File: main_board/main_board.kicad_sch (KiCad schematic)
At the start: 77 parts, among them J1 3.5mm Jack, J18 Conn_01x15_Female, J19 Conn_01x15_Female, J2 3.5mm Jack, J20 Conn_01x02_Male, J3 3.5mm Jack, J4 3.5mm Jack, J5 Display Header, J6 EU Power, J7 Expansion Header, SW1 Push Button, SW10 Push Button, SW11 Push Button, SW12 Push Button, SW13 Push Button, SW14 Push Button, SW15 Push Button, SW16 Push Button, SW17 Push Button, SW2 Push Button, SW3 Push Button, SW4 Push Button, SW5 Adj, SW6 Push Button, SW7 Push Button, SW8 Push Button, SW9 Push Button, U16 MB85RC256

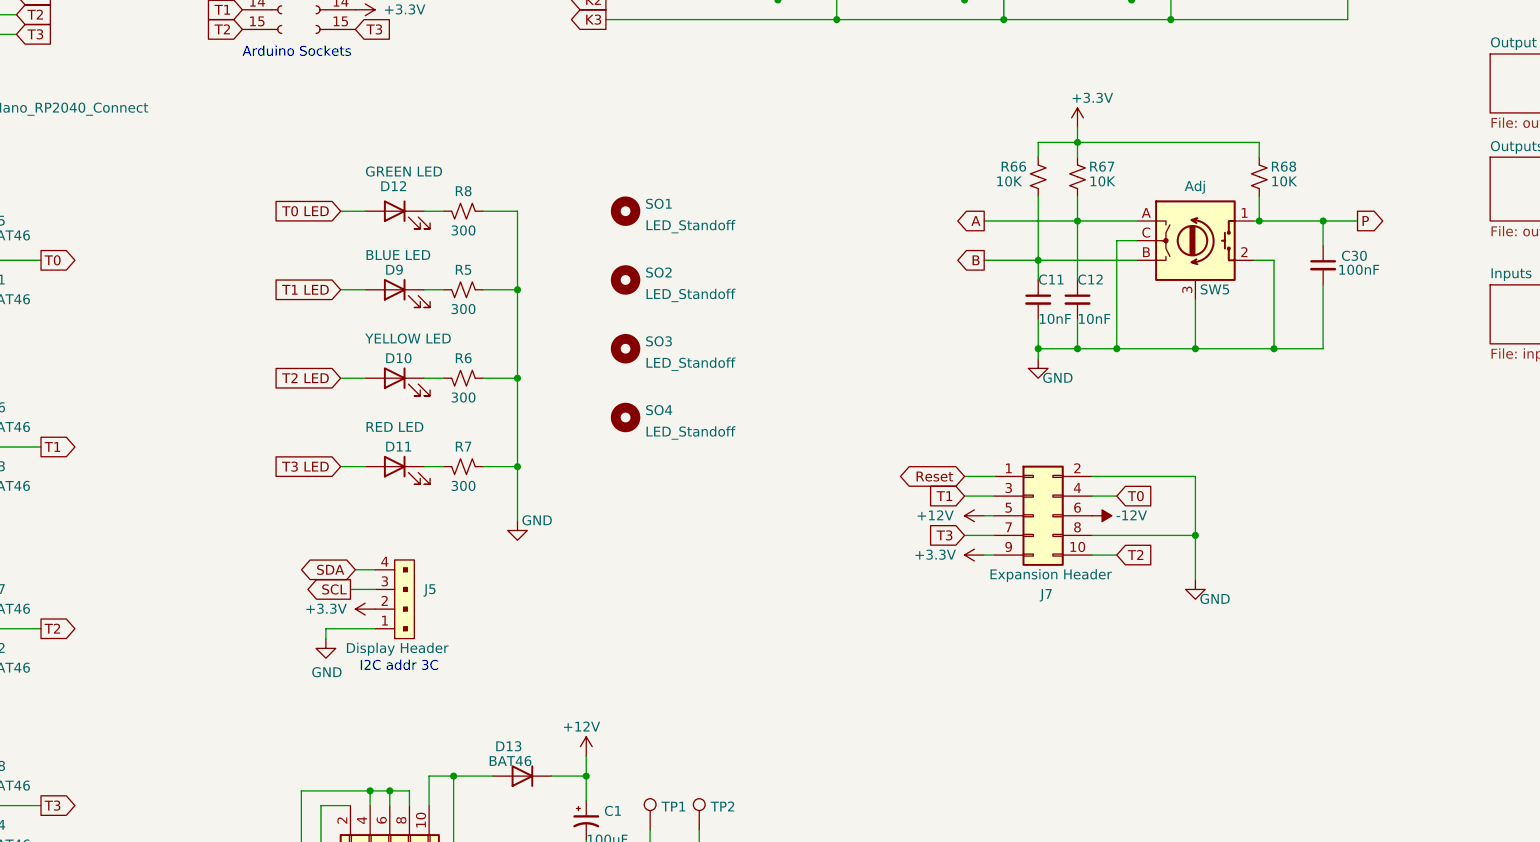
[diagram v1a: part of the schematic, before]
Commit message: Version .20
Moves to external library
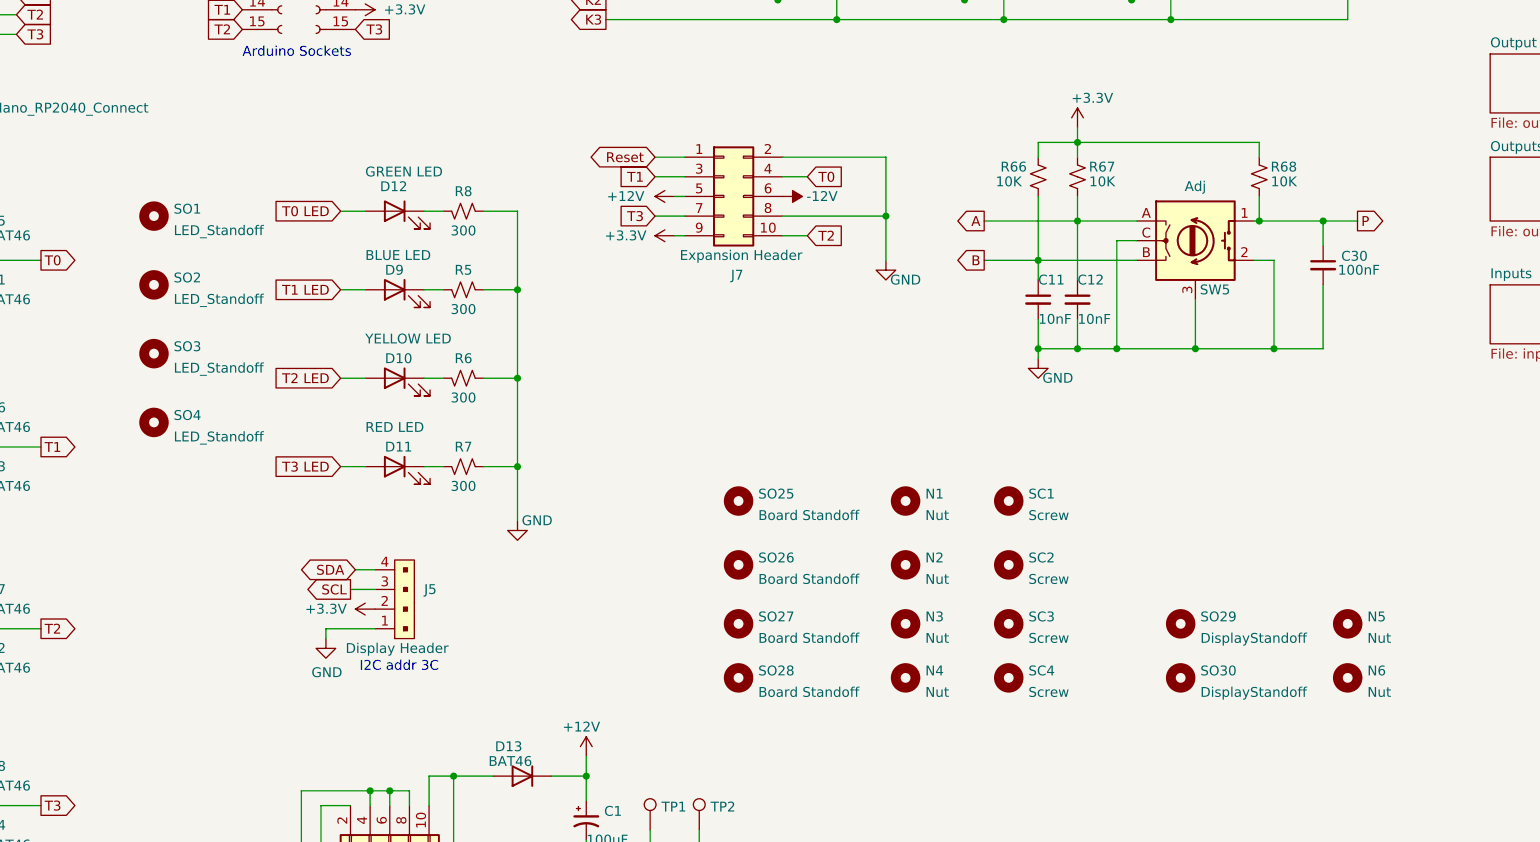
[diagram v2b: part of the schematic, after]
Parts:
- added N1, N2, N3, N4, N5, N6: Nut, symbol greenface:LED_Standoff
- added SC1, SC2, SC3, SC4: Screw, symbol greenface:LED_Standoff
- added SO25, SO26, SO27, SO28: Board Standoff, symbol greenface:LED_Standoff
- added SO29, SO30: DisplayStandoff, symbol greenface:LED_Standoff
- D10: Digi-Key Part 160-1035-ND -> 160-1961-ND
- D11: Digi-Key Part 160-1035-ND -> 732-5005-ND
- D12: Digi-Key Part 160-1035-ND -> 732-5008-ND
- D9: Digi-Key Part 160-1035-ND -> 732-11401-ND
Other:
- moved on the sheet: J7, SO1, SO2, SO3, SO4

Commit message: Software v2.2
Removes unneeded files.
Adds pre-flight handler in WiFi do_server();
Removes debug printouts.
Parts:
- J20:  LCSC Part # (none) -> C492401
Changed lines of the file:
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@@
+      (effects (font (size 1.27 1.27)) hide)
+    )
+    (property " LCSC Part #" "C492401" (id 5) (at 120.015 24.765 0)
       (effects (font (size 1.27 1.27)) hide)
     )
@@
     )
     (path "/eae55a42-d110-46e1-b06f-560b3d6a7f91/c48ee5e9-0cb9-42be-91f7-fd1b8daadc67"
-      (reference "R93") (unit 1) (value "56K") (footprint "Resistor_SMD:R_0805_2012Metric_Pad1.20x1.40mm_HandSolder")
+      (reference "R93") (unit 1) (value "100K") (footprint "Resistor_SMD:R_0805_2012Metric_Pad1.20x1.40mm_HandSolder")
     )
     (path "/eae55a42-d110-46e1-b06f-560b3d6a7f91/8f467469-5b59-49bc-9a45-5c4c02cfd83f"
-      (reference "R94") (unit 1) (value "56K") (footprint "Resistor_SMD:R_0805_2012Metric_Pad1.20x1.40mm_HandSolder")
+      (reference "R94") (unit 1) (value "100K") (footprint "Resistor_SMD:R_0805_2012Metric_Pad1.20x1.40mm_HandSolder")
     )
     (path "/eae55a42-d110-46e1-b06f-560b3d6a7f91/28bf7470-e1d2-4e98-a4b6-f98eb30a5a64"
-      (reference "R95") (unit 1) (value "56K") (footprint "Resistor_SMD:R_0805_2012Metric_Pad1.20x1.40mm_HandSolder")
+      (reference "R95") (unit 1) (value "100K") (footprint "Resistor_SMD:R_0805_2012Metric_Pad1.20x1.40mm_HandSolder")
     )
     (path "/eae55a42-d110-46e1-b06f-560b3d6a7f91/1e88784e-1b90-44c4-aa24-62abd646680b"
-      (reference "R96") (unit 1) (value "56K") (footprint "Resistor_SMD:R_0805_2012Metric_Pad1.20x1.40mm_HandSolder")
+      (reference "R96") (unit 1) (value "100K") (footprint "Resistor_SMD:R_0805_2012Metric_Pad1.20x1.40mm_HandSolder")
     )
     (path "/eae55a42-d110-46e1-b06f-560b3d6a7f91/af0f4f1e-590a-4e44-bb6f-03e1b7a33730"
@@
     )
     (path "/eae55a42-d110-46e1-b06f-560b3d6a7f91/5392f86f-026a-44a3-8a1d-a0c922c48ed1"
-      (reference "R121") (unit 1) (value "56K") (footprint "Resistor_SMD:R_0805_2012Metric_Pad1.20x1.40mm_HandSolder")
+      (reference "R121") (unit 1) (value "100K") (footprint "Resistor_SMD:R_0805_2012Metric_Pad1.20x1.40mm_HandSolder")
     )
     (path "/eae55a42-d110-46e1-b06f-560b3d6a7f91/d5a79db5-b8c5-4dbc-8d68-88add333d998"
-      (reference "R122") (unit 1) (value "56K") (footprint "Resistor_SMD:R_0805_2012Metric_Pad1.20x1.40mm_HandSolder")
+      (reference "R122") (unit 1) (value "100K") (footprint "Resistor_SMD:R_0805_2012Metric_Pad1.20x1.40mm_HandSolder")
     )
     (path "/eae55a42-d110-46e1-b06f-560b3d6a7f91/758ac2e7-692f-4be8-92b8-a60d9b85da79"
-      (reference "R123") (unit 1) (value "56K") (footprint "Resistor_SMD:R_0805_2012Metric_Pad1.20x1.40mm_HandSolder")
+      (reference "R123") (unit 1) (value "100K") (footprint "Resistor_SMD:R_0805_2012Metric_Pad1.20x1.40mm_HandSolder")
     )
     (path "/eae55a42-d110-46e1-b06f-560b3d6a7f91/3d08366c-664c-49aa-9264-fe38e52d7908"
-      (reference "R124") (unit 1) (value "56K") (footprint "Resistor_SMD:R_0805_2012Metric_Pad1.20x1.40mm_HandSolder")
+      (reference "R124") (unit 1) (value "100K") (footprint "Resistor_SMD:R_0805_2012Metric_Pad1.20x1.40mm_HandSolder")
     )
     (path "/b12871f3-737e-47b7-9f4c-ecb6eabe1783"
@@
     )
     (path "/808a57ff-0ced-4535-b028-9fea6b6c5f09/36580576-1e78-433f-b141-eb68f497b9e6"
-      (reference "R139") (unit 1) (value "56K") (footprint "Resistor_SMD:R_0805_2012Metric_Pad1.20x1.40mm_HandSolder")
+      (reference "R139") (unit 1) (value "100K") (footprint "Resistor_SMD:R_0805_2012Metric_Pad1.20x1.40mm_HandSolder")
     )
     (path "/808a57ff-0ced-4535-b028-9fea6b6c5f09/b8029def-cd05-4fce-a794-515779c7678d"
-      (reference "R140") (unit 1) (value "56K") (footprint "Resistor_SMD:R_0805_2012Metric_Pad1.20x1.40mm_HandSolder")
+      (reference "R140") (unit 1) (value "100K") (footprint "Resistor_SMD:R_0805_2012Metric_Pad1.20x1.40mm_HandSolder")
     )
     (path "/b200c1d4-b772-4a0d-a7bc-c10bcb241496/fce33d75-d8cb-456f-b73c-6382e195250c"
